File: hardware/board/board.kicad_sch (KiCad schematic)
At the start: 126 parts, among them J2 Conn_01x26_MountingPin, J3 Conn_01x26_MountingPin, J4 Conn_01x26_MountingPin, J5 Conn_01x03, SW1 SW_Push, SW2 SW_Push, SW3 SKRTLAE010, U1 STM32WB55RGV6, U10 74HC4051, U11 74HC4051, U12 74HC4051, U13 SN74LV1T125DCKR, U14 USBLC6-2P6, U15 FAN48610BUC50X, U16 RS3221-3.3YUTDN4, U7 74HC4051, U8 74HC4051, U9 74HC4051, X1 XL7EL89CKI-111YLC-32M, X2 FC-12M32.768KHZ7PF20PPM

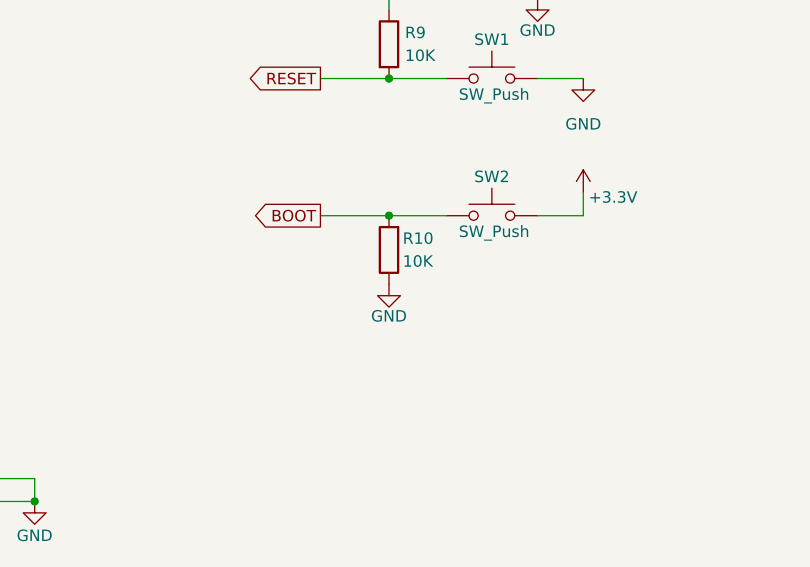
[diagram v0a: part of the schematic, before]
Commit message: impdance matching
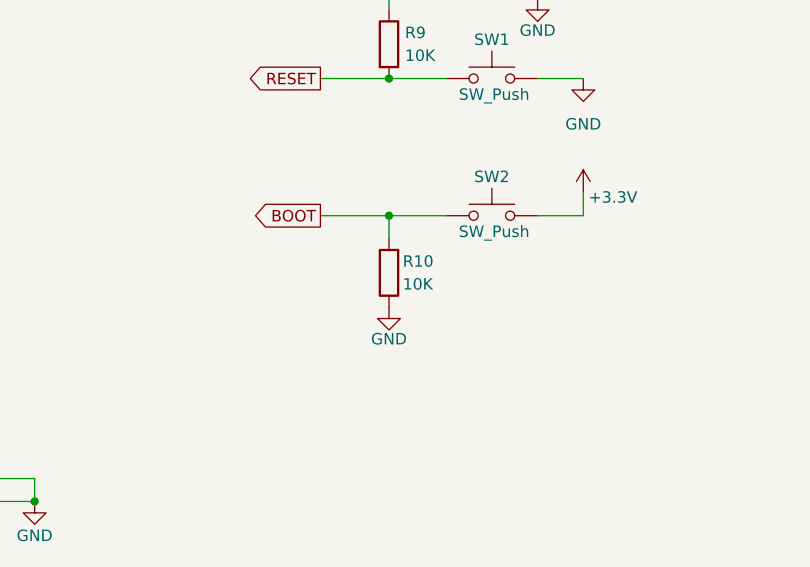
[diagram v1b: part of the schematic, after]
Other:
- moved on the sheet: R10
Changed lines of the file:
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@@
 	(wire
 		(pts
+			(xy 251.46 151.13) (xy 251.46 148.59)
+		)
+		(stroke
+			(width 0)
+			(type default)
+		)
+	)
+	(wire
+		(pts
 			(xy 162.56 66.04) (xy 166.37 66.04)
 		)
@@
 	(symbol
 		(lib_id "power:GND")
-		(at 251.46 156.21 0)
+		(at 251.46 158.75 0)
 		(unit 1)
 		(exclude_from_sim no)
@@
 		(dnp no)
 		(property "Reference" "#PWR028"
-			(at 251.46 162.56 0)
+			(at 251.46 165.1 0)
 			(effects
 				(font
@@
 		)
 		(property "Value" "GND"
-			(at 251.46 159.766 0)
+			(at 251.46 162.306 0)
 			(effects
 				(font
@@
 		)
 		(property "Footprint" ""
-			(at 251.46 156.21 0)
+			(at 251.46 158.75 0)
 			(effects
 				(font
@@
 		)
 		(property "Datasheet" ""
-			(at 251.46 156.21 0)
+			(at 251.46 158.75 0)
 			(effects
 				(font
@@
 		)
 		(property "Description" "Power symbol creates a global label with name \"GND\" , ground"
-			(at 251.46 156.21 0)
+			(at 251.46 158.75 0)
 			(effects
 				(font
@@
 	(symbol
 		(lib_id "Device:R")
-		(at 251.46 152.4 180)
+		(at 251.46 154.94 180)
 		(unit 1)
 		(exclude_from_sim no)
@@
 		(dnp no)
 		(property "Reference" "R10"
-			(at 252.984 151.13 0)
+			(at 252.984 153.67 0)
 			(effects
 				(font
@@
 		)
 		(property "Value" "10K"
-			(at 252.984 153.67 0)
+			(at 252.984 156.21 0)
 			(effects
 				(font
@@
 		)
 		(property "Footprint" "Resistor_SMD:R_0402_1005Metric"
-			(at 253.238 152.4 90)
+			(at 253.238 154.94 90)
 			(effects
 				(font
@@
 		)
 		(property "Datasheet" "~"
-			(at 251.46 152.4 0)
+			(at 251.46 154.94 0)
 			(effects
 				(font
@@
 		)
 		(property "Description" "Resistor"
-			(at 251.46 152.4 0)
+			(at 251.46 154.94 0)
 			(effects
 				(font
